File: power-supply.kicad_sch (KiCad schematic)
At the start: 2 parts, among them U6 TPS61230DRC, U7 LM3670MF

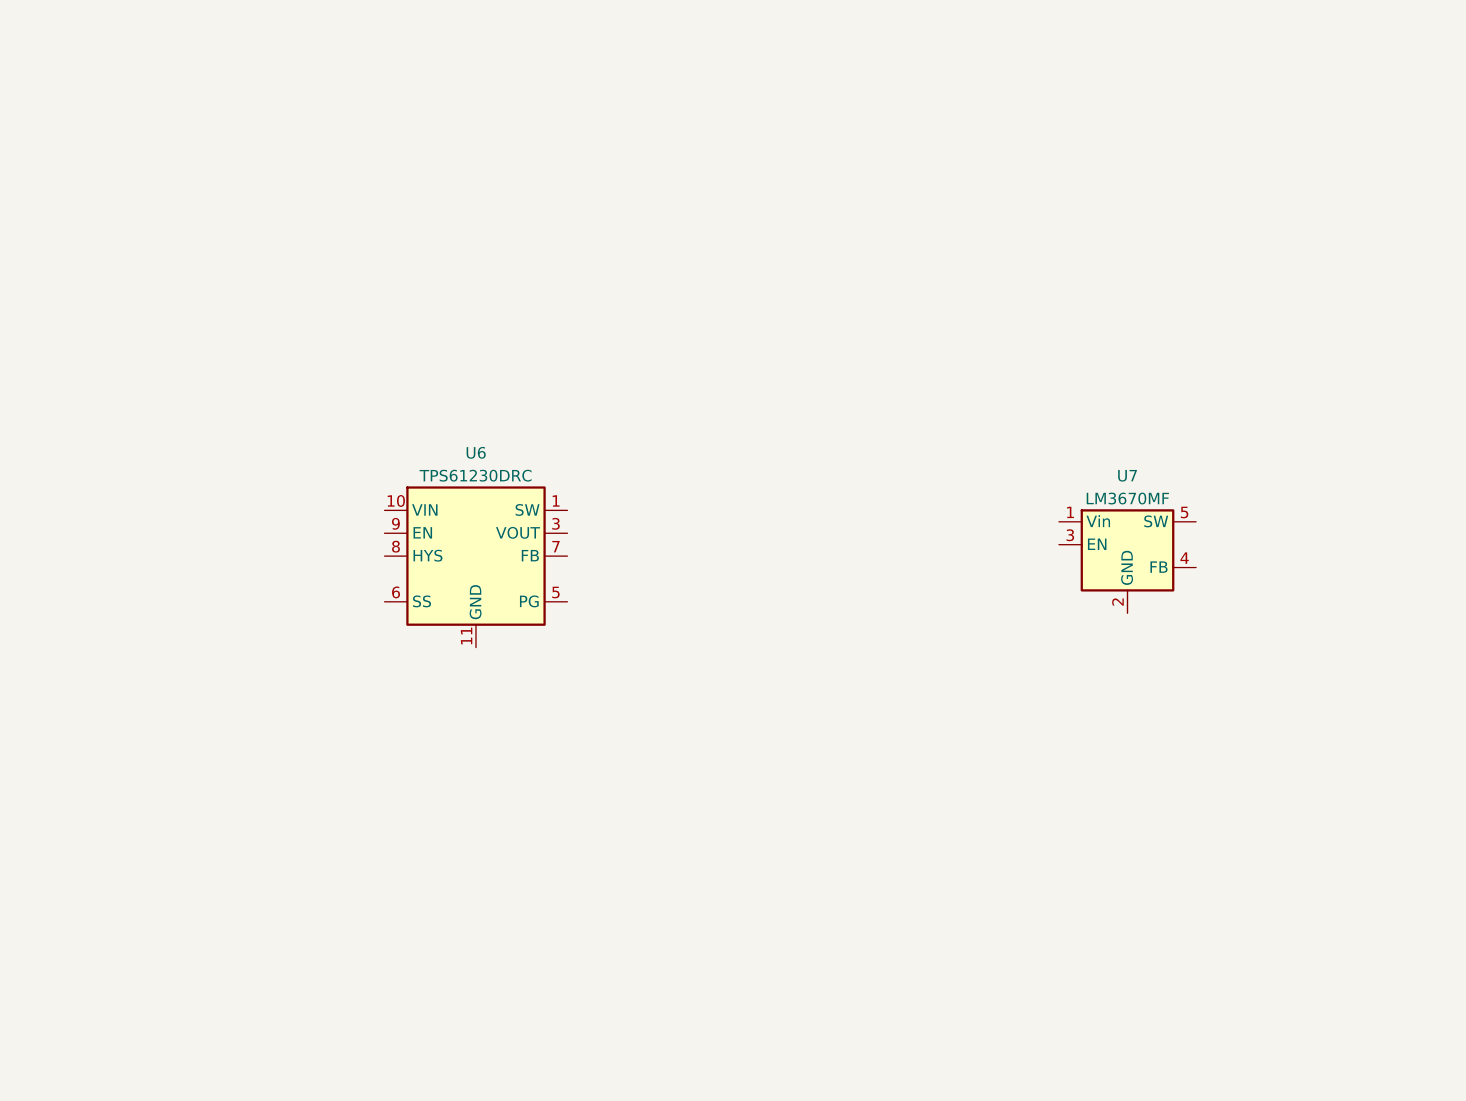
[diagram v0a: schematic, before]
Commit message: Added power supply circuitry, as well as example pyrotechnic channel MOSFET
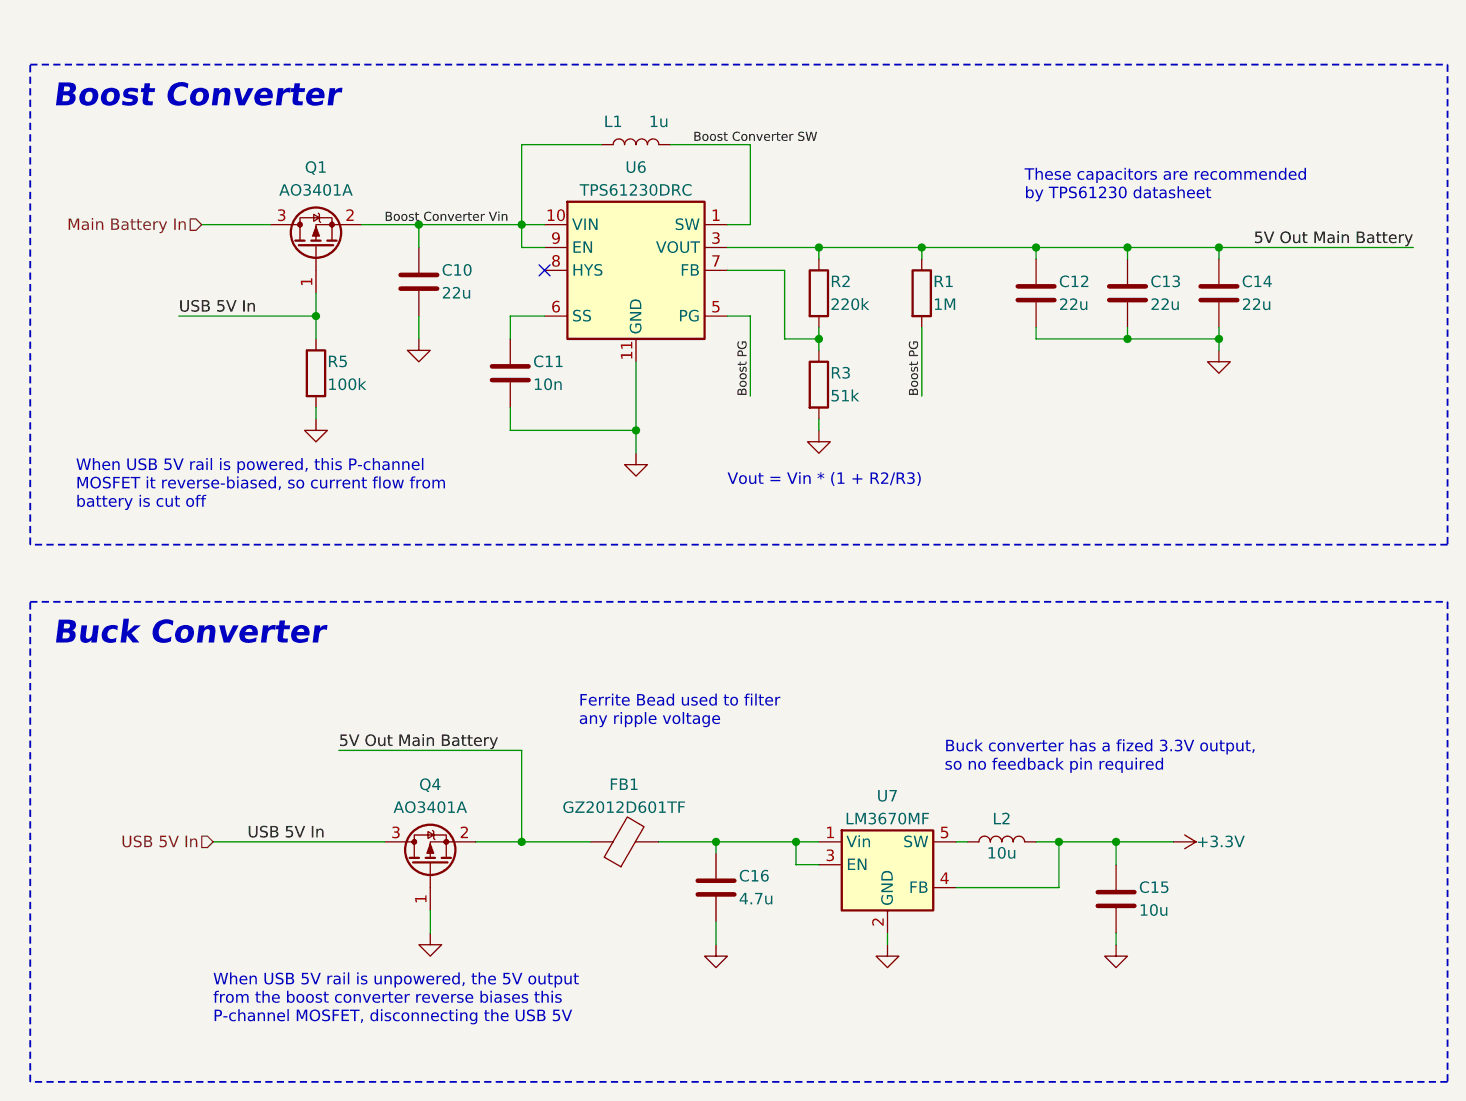
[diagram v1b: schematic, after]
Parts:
- added C10, C12, C13, C14: 22u, symbol Device:C
- added C11: 10n, symbol Device:C
- added C15: 10u, symbol Device:C
- added C16: 4.7u, symbol Device:C
- added FB1: GZ2012D601TF, symbol Device:FerriteBead
- added L1: 1u, symbol Device:L
- added L2: 10u, symbol Device:L
- added Q1, Q4: AO3401A, Package_TO_SOT_SMD:SOT-23, symbol Transistor_FET:AO3401A
- added R1: 1M, symbol Device:R
- added R2: 220k, symbol Device:R
- added R3: 51k, symbol Device:R
- added R5: 100k, symbol Device:R
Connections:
- net at U7.1 (Vin): now also U7.3 (EN), C16.1, FB1.2
- net GND: now reaches U7.2 (GND)
- net GND: now also U6.11 (GND), C10.2, C11.2, C12.2, C13.2, C14.2, C15.2, C16.2, Q4.1 (G), R3.2, R5.2
- net +3.3V: now reaches U7.4 (FB)
- net +3.3V: now also C15.1, L2.2
- net at U7.5 (SW): now also L2.1
- net Boost Converter SW: now reaches U6.1 (SW), U6.2 (SW)
- net Boost Converter SW: now also L1.2
- net Boost Converter Vin: now reaches U6.10 (VIN)
- net Boost Converter Vin: now also U6.9 (EN), C10.1, L1.1, Q1.2 (S)
- net 5V Out Main Battery: now reaches U6.3 (VOUT), U6.4 (VOUT)
- net 5V Out Main Battery: now also C12.1, C13.1, C14.1, FB1.1, Q4.2 (S), R1.1, R2.1
- net Boost PG: now reaches U6.5 (PG)
- net Boost PG: now also R1.2
- net at U6.6 (SS): now also C11.1
- net at U6.7 (FB): now also R2.2, R3.1
- new net Main Battery In: Q1.3 (D)
- new net USB 5V In: Q1.1 (G), Q4.3 (D), R5.1
- no-connect marks 0 -> 1
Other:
- note added: "Boost Converter"
- note added: "Buck Converter"
- note added: "Buck converter has a fized 3.3V output, so no feedback pin required"
- note added: "Ferrite Bead used to filter any ripple voltage"
- note added: "These capacitors are recommended by TPS61230 datasheet"
- note added: "Vout = Vin * (1 + R2/R3)"
- note added: "When USB 5V rail is powered, this P-channel MOSFET it reverse-biased, so current flow from battery is cut off"
- note added: "When USB 5V rail is unpowered, the 5V output from the boost converter reverse biases this P-channel MOSFET, disconnecting the USB 5V"
- moved on the sheet: U6, U7

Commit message: How many sheets do you want? Yes
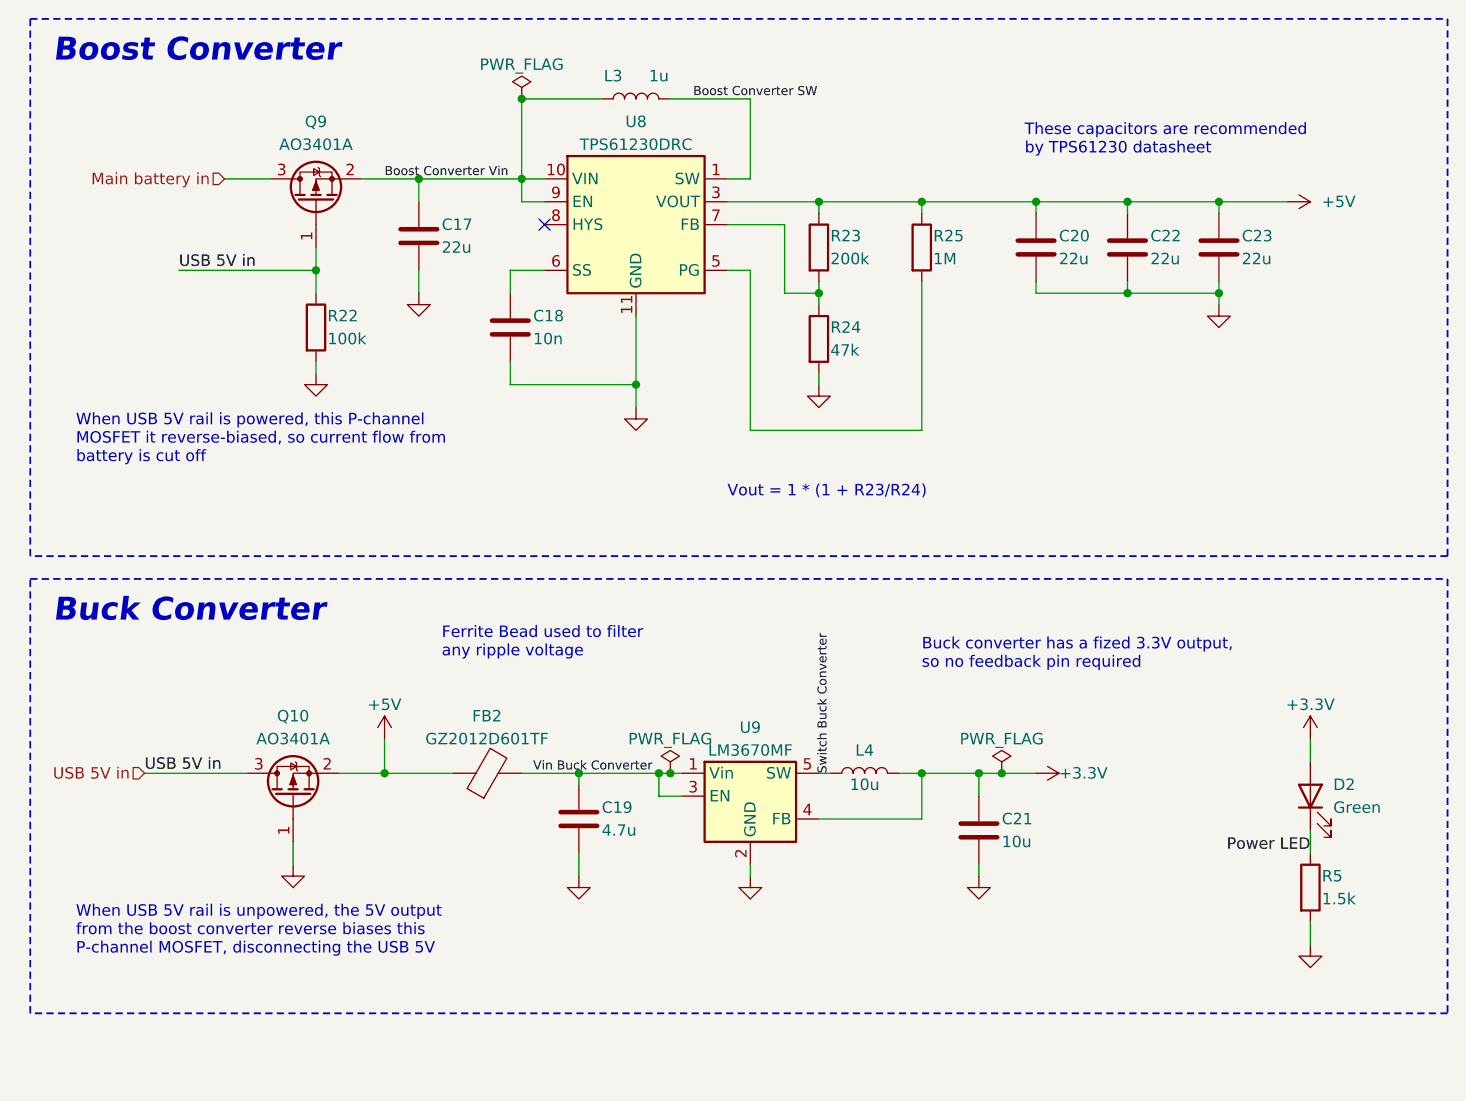
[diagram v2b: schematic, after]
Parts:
- removed C10, C12, C13, C14: 22u, symbol Device:C
- removed C11: 10n, symbol Device:C
- removed C15: 10u, symbol Device:C
- removed C16: 4.7u, symbol Device:C
- removed FB1: GZ2012D601TF, symbol Device:FerriteBead
- removed L1: 1u, symbol Device:L
- removed L2: 10u, symbol Device:L
- removed Q1, Q4: AO3401A, Package_TO_SOT_SMD:SOT-23, symbol Transistor_FET:AO3401A
- removed R1: 1M, symbol Device:R
- removed R2: 220k, symbol Device:R
- removed R3: 51k, symbol Device:R
- removed U6: TPS61230DRC, Package_SON:Texas_S-PVSON-N10_ThermalVias, symbol Regulator_Switching:TPS61230DRC
- removed U7: LM3670MF, Package_TO_SOT_SMD:TSOT-23-5, symbol Regulator_Switching:LM3670MF
- added C17, C20, C22, C23: 22u, Capacitor_SMD:C_0805_2012Metric, symbol Device:C
- added C18: 10n, Capacitor_SMD:C_0402_1005Metric, symbol Device:C
- added C19: 4.7u, Capacitor_SMD:C_0603_1608Metric, symbol Device:C
- added C21: 10u, Capacitor_SMD:C_0805_2012Metric, symbol Device:C
- added D2: Green, LED_SMD:LED_0805_2012Metric, symbol Device:LED
- added FB2: GZ2012D601TF, Inductor_SMD:L_0805_2012Metric, symbol Device:FerriteBead
- added L3: 1u, Inductor_SMD:L_Sunlord_SWPA4030S, symbol Device:L
- added L4: 10u, Inductor_SMD:L_Sunlord_SWPA4030S, symbol Device:L
- added Q10, Q9: AO3401A, Package_TO_SOT_SMD:SOT-23, symbol Transistor_FET:AO3401A
- added R22: 100k, Resistor_SMD:R_0402_1005Metric, symbol Device:R
- added R23: 200k, Resistor_SMD:R_0402_1005Metric, symbol Device:R
- added R24: 47k, Resistor_SMD:R_0402_1005Metric, symbol Device:R
- added R25: 1M, Resistor_SMD:R_0402_1005Metric, symbol Device:R
- added U8: TPS61230DRC, Package_SON:Texas_S-PVSON-N10_ThermalVias, symbol Regulator_Switching:TPS61230DRC
- added U9: LM3670MF, Package_TO_SOT_SMD:TSOT-23-5, symbol Regulator_Switching:LM3670MF
- R5: value 100k -> 1.5k; footprint (none) -> Resistor_SMD:R_0603_1608Metric
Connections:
- net +3.3V: now also C21.1, D2.2 (A), L4.2, U9.4 (FB)
- net Boost Converter SW: now also L3.2, U8.1 (SW), U8.2 (SW)
- net Boost Converter Vin: now also C17.1, L3.1, Q9.2 (S), U8.10 (VIN), U8.9 (EN)
- net GND: now also C17.2, C18.2, C19.2, C20.2, C21.2, C22.2, C23.2, Q10.1 (G), R22.2, R24.2, U8.11 (GND), U9.2 (GND)
- net USB 5V In renamed Power LED
- net Power LED: now also D2.1 (K)
- new net: R25.2, U8.5 (PG)
- new net: C18.1, U8.6 (SS)
- new net: R23.2, R24.1, U8.7 (FB)
- new net +5V: C20.1, C22.1, C23.1, FB2.1, Q10.2 (S), R23.1, R25.1, U8.3 (VOUT), U8.4 (VOUT)
- new net Main battery in: Q9.3 (D)
- new net Switch Buck Converter: L4.1, U9.5 (SW)
- new net USB 5V in: Q10.3 (D), Q9.1 (G), R22.1
- new net Vin Buck Converter: C19.1, FB2.2, U9.1 (Vin), U9.3 (EN)
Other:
- note added: "Vout = 1 * (1 + R23/R24)"
- note removed: "Vout = Vin * (1 + R2/R3)"
